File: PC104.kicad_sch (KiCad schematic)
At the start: 10 parts

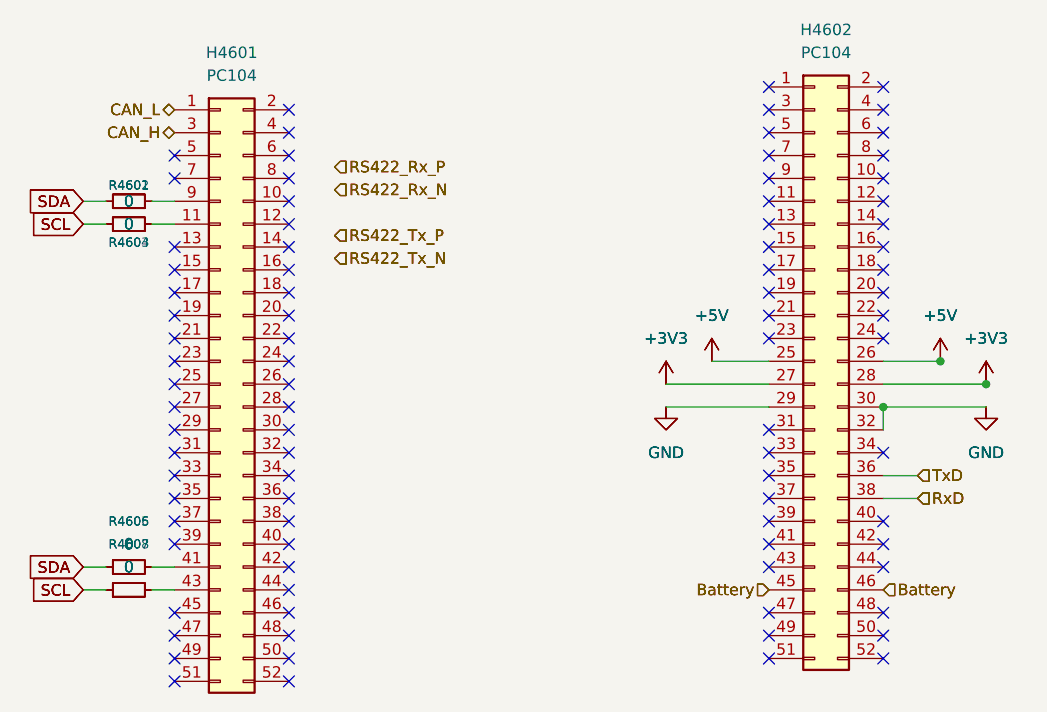
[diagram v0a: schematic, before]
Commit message: progress on CORE pcb
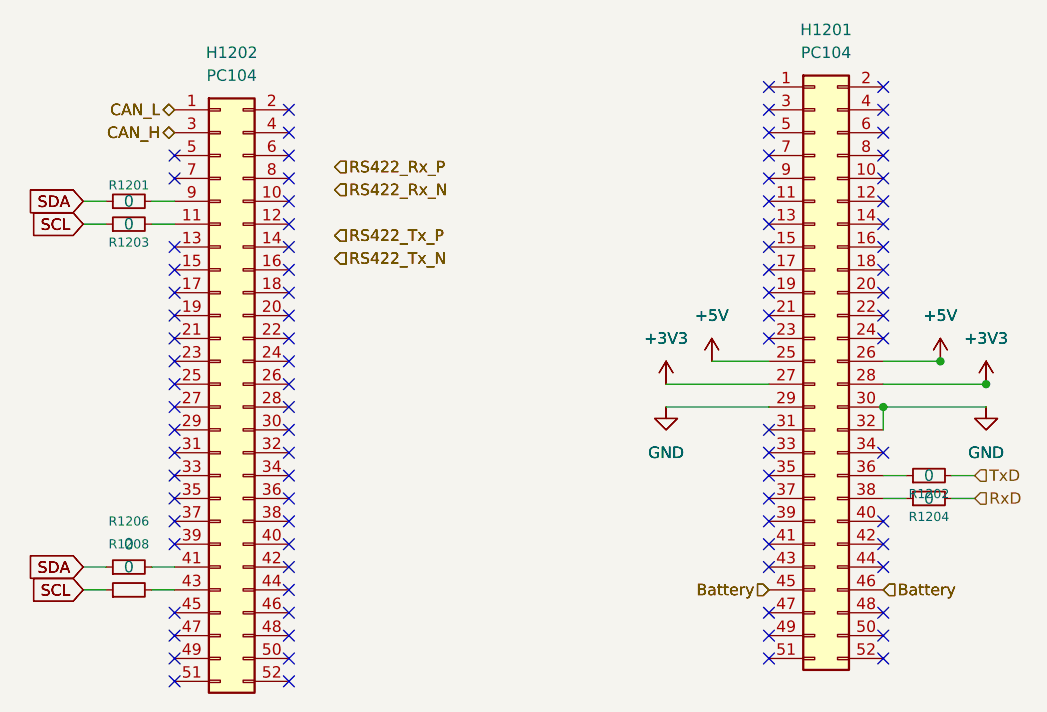
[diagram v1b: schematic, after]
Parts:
- removed R4602, R4604, R4605, R4607: 0, Resistor_SMD:R_0603_1608Metric_Pad0.98x0.95mm_HandSolder, symbol Device:R_Small
- added R1202, R1204: 0, Resistor_SMD:R_0603_1608Metric_Pad0.98x0.95mm_HandSolder, symbol Device:R_Small
- renumbered H4602 to H1201, H4601 to H1202, R4601 to R1201, R4603 to R1203, R4606 to R1206, R4608 to R1208
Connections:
- net RxD: now also R1204.2; no longer H1201.38 (Pin_38)
- net TxD: now also R1202.2; no longer H1201.36 (Pin_36)
- new net: H1201.38 (Pin_38), R1204.1
- new net: H1201.36 (Pin_36), R1202.1
